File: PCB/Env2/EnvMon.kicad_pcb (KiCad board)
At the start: 2 copper layers, 70 x 70 mm, 51 parts, among them J1 LCD, J10 Conn_01x01, J11 Conn_01x01, J12 Conn_01x01, J2 DC, J3 TEMP, J4 LCD, J5 Reset, J6 USB-C-Socket-H, J7 TC2030-USB-NL-DS, J8 T6793, J9 Conn_01x01, U1 ESP32-S3-MINI-1, U2 SCD41, U3 MD8942, U4 MCP9808_MSOP, U5 GZP6816D, U8 VEML6040

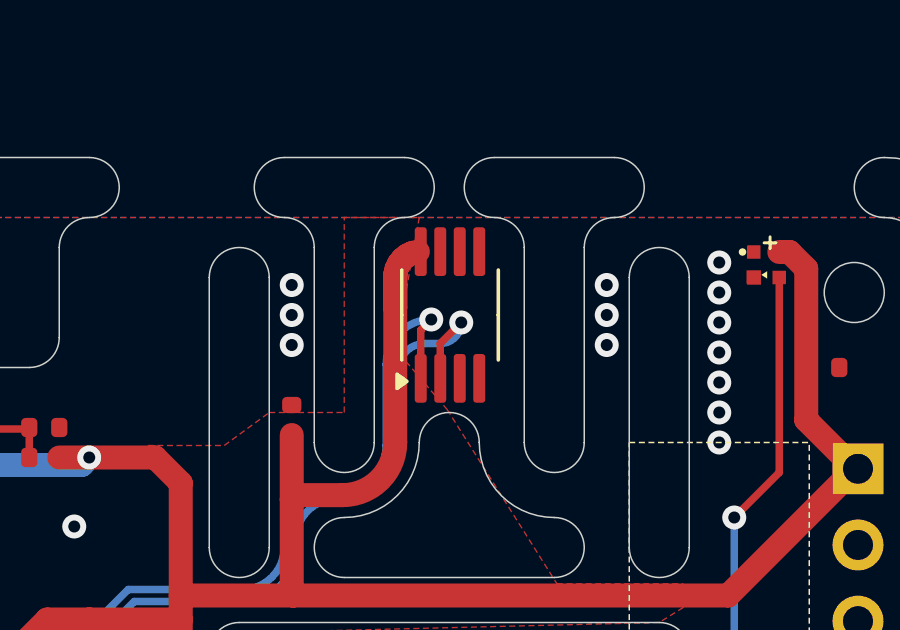
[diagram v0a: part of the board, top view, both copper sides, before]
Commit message: New case work
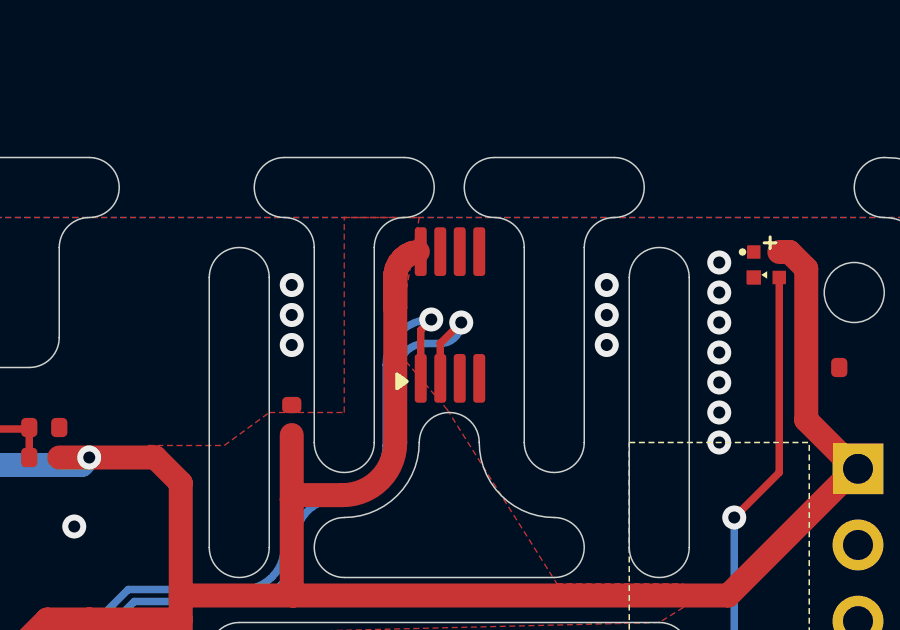
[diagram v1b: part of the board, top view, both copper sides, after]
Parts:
- D4: footprint RevK:SMD1010-Side -> RevK:SMD1010-Side2
- U4: footprint Package_SO:MSOP-8_3x3mm_P0.65mm -> RevK:MSOP-8_3x3mm_P0.65mm-SIde

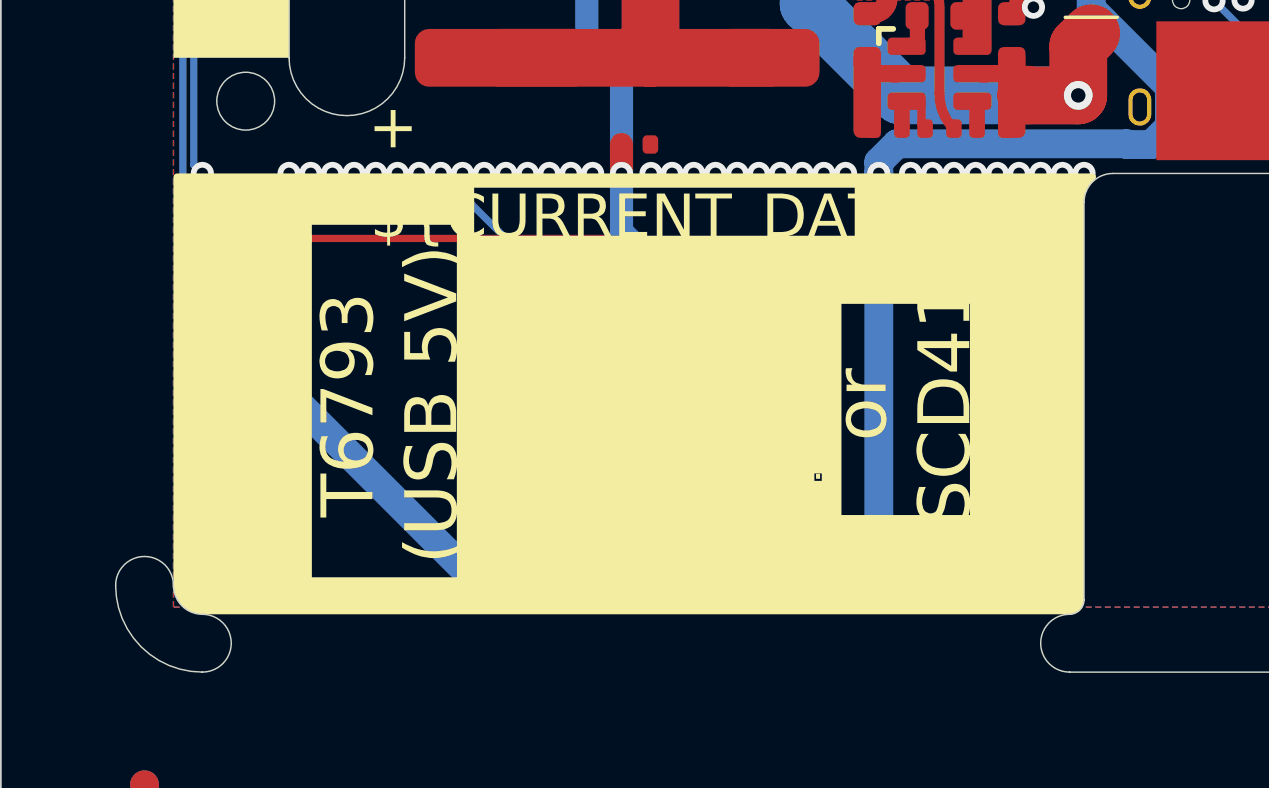
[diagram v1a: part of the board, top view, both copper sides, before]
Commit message: Library update
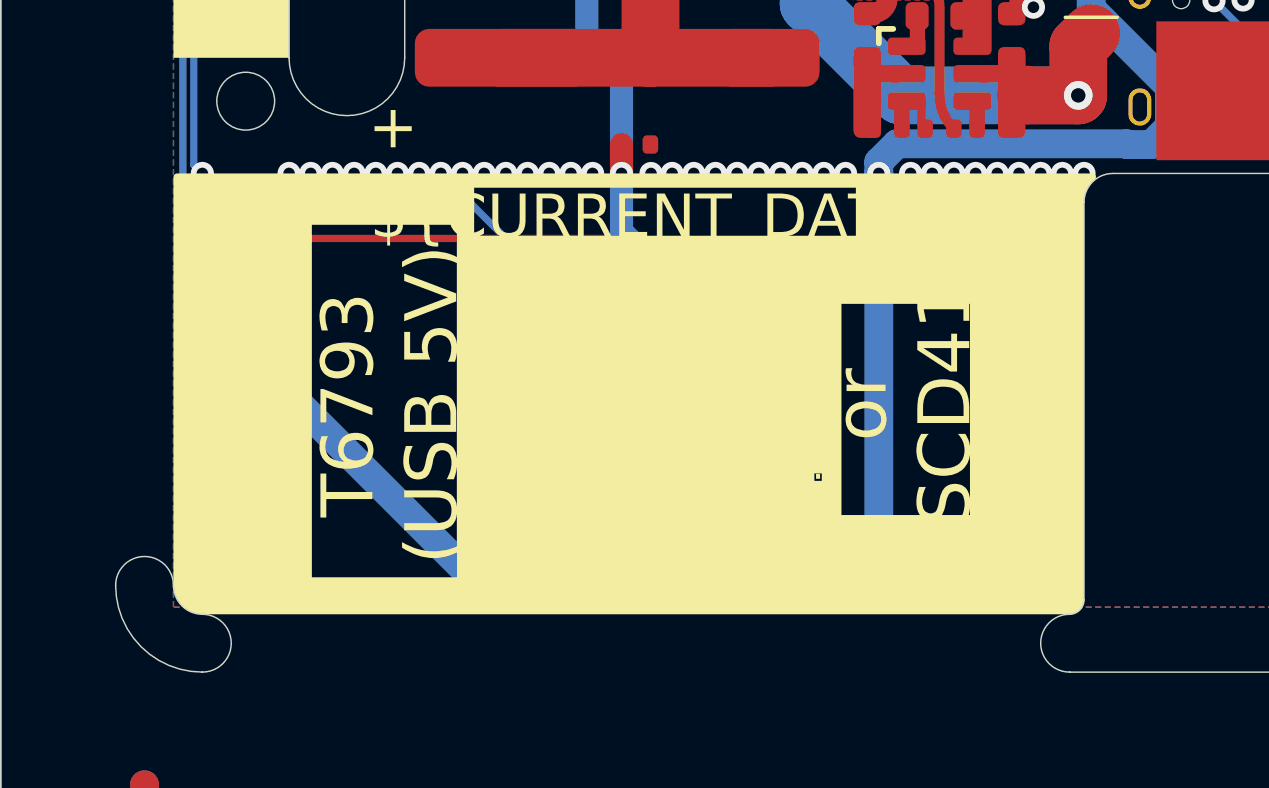
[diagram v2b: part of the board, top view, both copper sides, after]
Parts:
- moved J1 28.0 mm to (100.0, 92.5)
